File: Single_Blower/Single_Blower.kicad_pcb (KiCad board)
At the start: 2 copper layers, 70 x 65 mm, 17 parts, among them J1 BLOWER, J3 LED, J4 Sensor Connection, J5 LIMIT Switch, J6 DE9_Pins_MountingHoles, U2 5V

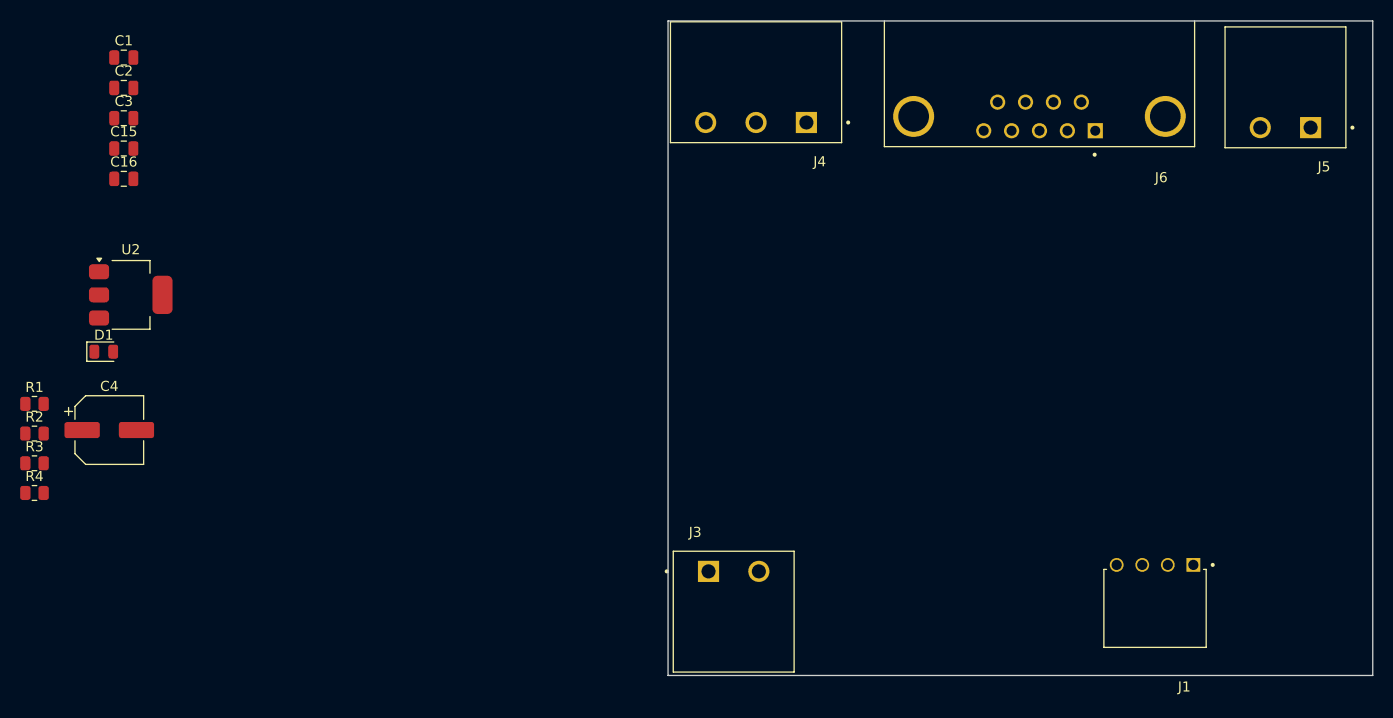
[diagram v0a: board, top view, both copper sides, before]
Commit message: Finished routing single blower
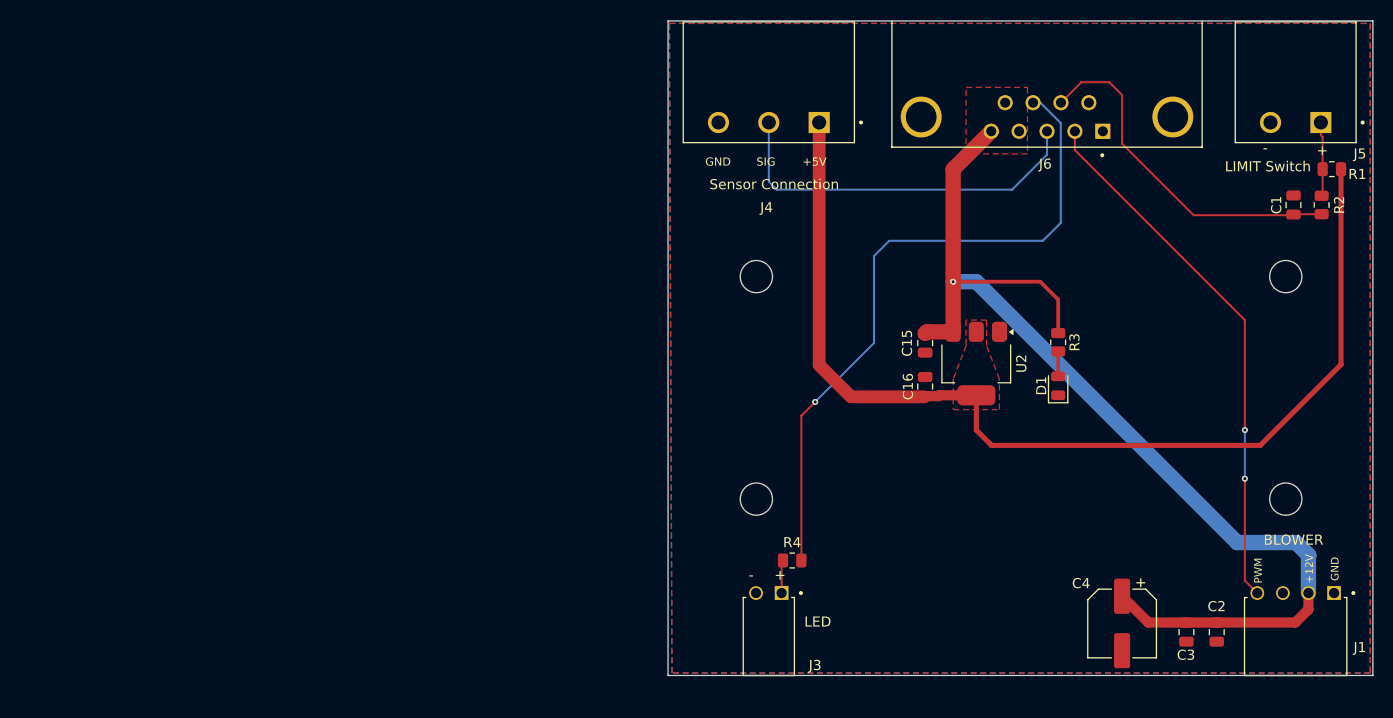
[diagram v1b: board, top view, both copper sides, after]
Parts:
- added H1: MountingHole, MountingHole:MountingHole_3.2mm_M3_DIN965, F.Cu at (130.0, 59.9)
- added H2: MountingHole, MountingHole:MountingHole_3.2mm_M3_DIN965, F.Cu at (182.6, 59.9)
- added H3: MountingHole, MountingHole:MountingHole_3.2mm_M3_DIN965, F.Cu at (182.6, 82.0)
- added H4: MountingHole, MountingHole:MountingHole_3.2mm_M3_DIN965, F.Cu at (130.0, 82.0)
- J3: footprint Single_blower_footprints:PHOENIX_1923759 -> Single_blower_footprints:TE_640457-2
- moved R1 130.9 mm to (187.2, 49.3), turned to 180 degrees
- moved R2 129.8 mm to (186.2, 52.8), turned to 90 degrees
- moved C2 121.3 mm to (175.8, 95.2), turned to -90 degrees
- moved C3 117.2 mm to (172.8, 95.2), turned to -90 degrees
- moved C1 117.1 mm to (183.4, 52.8), turned to 90 degrees
- moved C4 102.4 mm to (166.4, 94.4), turned to -90 degrees
- moved R3 102.4 mm to (160.0, 66.5), turned to -90 degrees
- moved D1 94.8 mm to (160.0, 70.8), turned to 90 degrees
- moved U2 84.3 mm to (151.9, 68.6), turned to -90 degrees
- moved C16 82.2 mm to (146.8, 70.9), turned to 90 degrees
- moved C15 81.9 mm to (146.8, 66.5), turned to -90 degrees
- moved R4 75.5 mm to (133.6, 88.1), turned to 180 degrees
- moved J1 14.2 mm to (187.4, 91.4)
- moved J3 13.3 mm to (132.6, 91.4), turned to 180 degrees
- moved J4 1.27 mm to (139.8, 34.6)
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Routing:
- net +12V: track 0.00 -> 110.9 mm, vias 0 -> 1
- net +5V: track 0.00 -> 104.4 mm
- net LED_PIN: track 0.00 -> 66.6 mm, vias 0 -> 1
- net PWM_PIN: track 0.00 -> 53.4 mm, vias 0 -> 2
- net SENSOR_PIN: track 0.00 -> 37.6 mm
- net LIMIT_PIN: track 0.00 -> 35.1 mm
- net Net-(J5-Pin_1): track 0.00 -> 7.40 mm
- net Net-(J3-Pin_1): track 0.00 -> 3.29 mm
- net Net-(D1-A): track 0.00 -> 2.47 mm
- added copper zone on F.Cu, net +12V
- added copper zone on F.Cu, net +5V
- added copper zone on B.Cu, net GND
- added copper zone on F.Cu, net GND
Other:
- board text added: "+"
- board text added: "+12V"
- board text added: "+5V"
- board text added: "-"
- board text added: "GND"
- board text added: "PWM"
- board text added: "SIG"
